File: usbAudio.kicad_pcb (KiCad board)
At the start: 2 copper layers, 34 parts, among them J2 USB_C_Receptacle_USB2.0_14P, J3 AudioJack3, SW1 PLAY/PAUSE, SW4 VOL+, SW5 VOL-, SW8 SW_SPDT, U1 PCM2706CPJTR, U4 MIC5504-3.3YM5-TR, Y2 Crystal_GND24

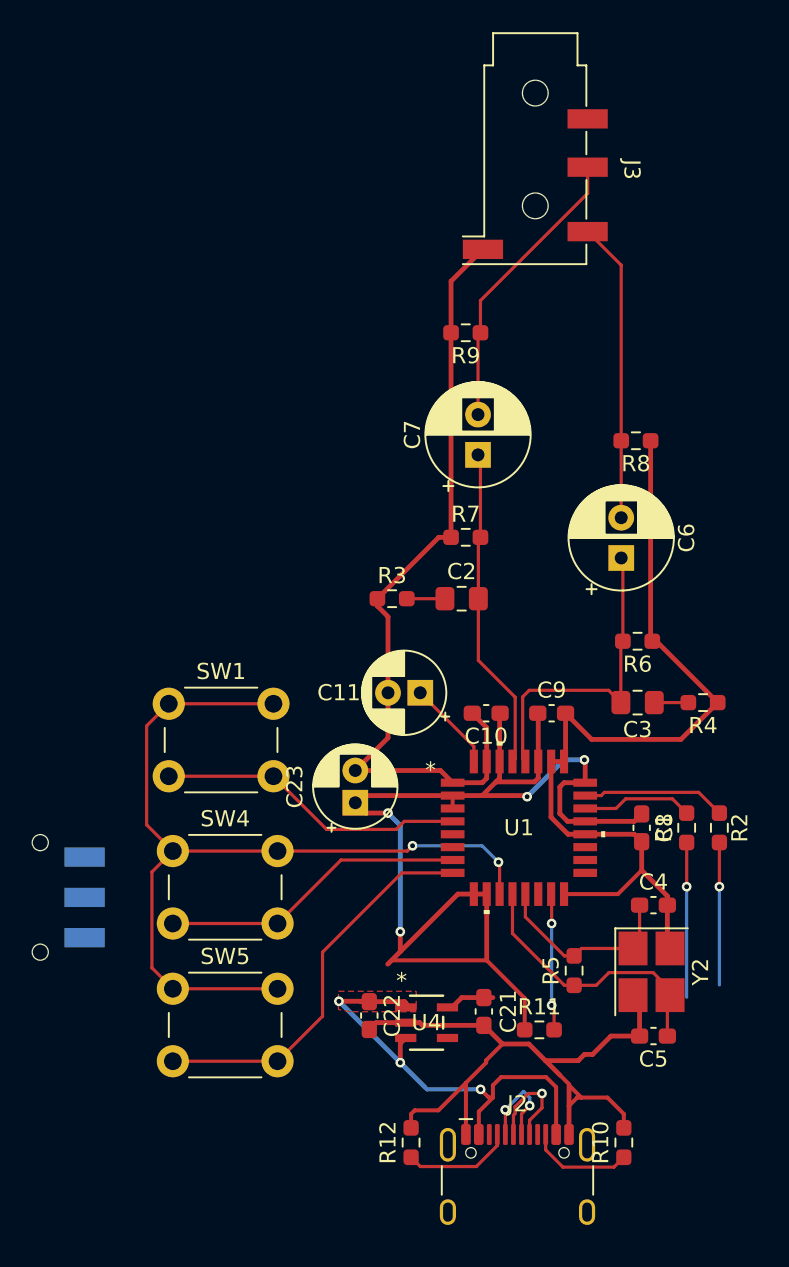
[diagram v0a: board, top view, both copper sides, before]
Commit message: Made ready for production!
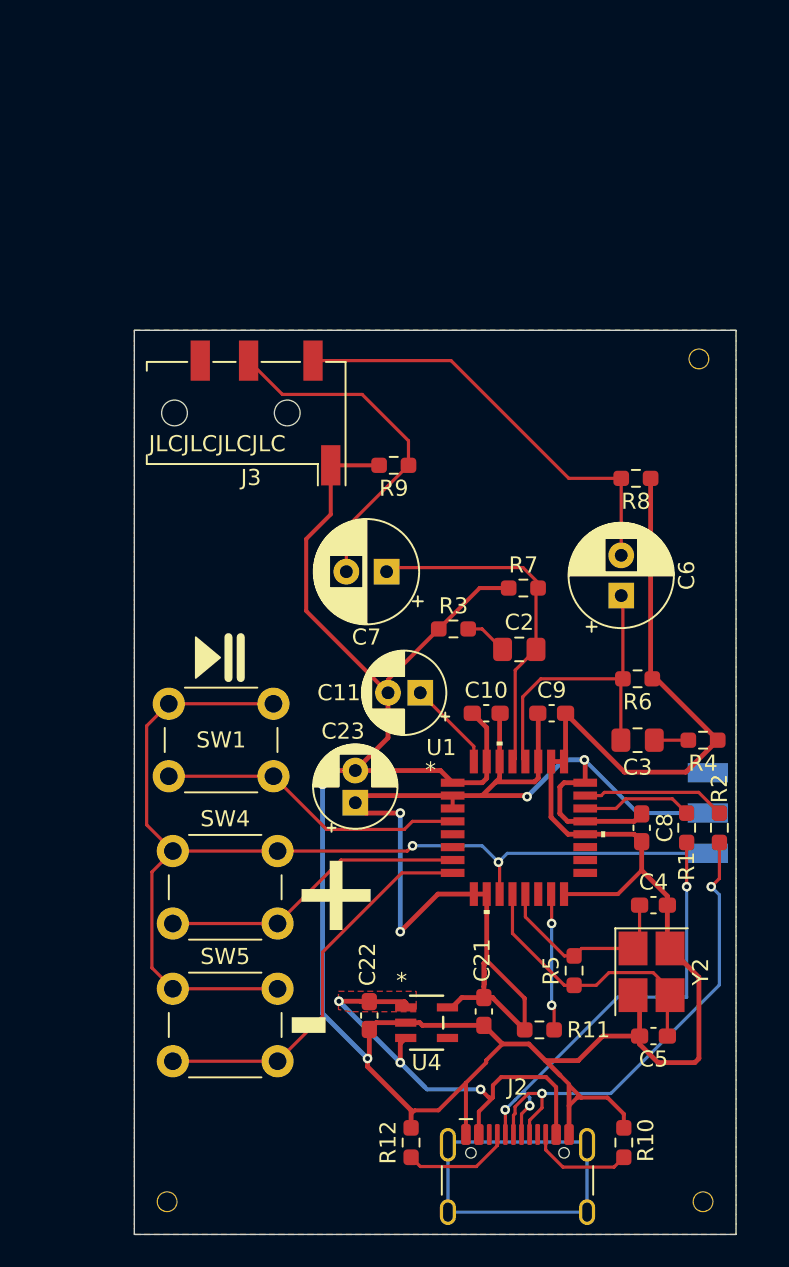
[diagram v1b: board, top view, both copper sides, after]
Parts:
- added G***: LOGO, LOGO, B.Cu at (141.4, 71.3)
- added G***: LOGO, LOGO, B.Cu at (126.0, 74.9)
- added G***: LOGO, LOGO, B.Cu at (141.0, 97.3)
- added REF**: PCBA tooling hole, JLCtooling:PCBA tooling hole, F.Cu at (119.4, 114.8)
- added REF**: PCBA tooling hole, JLCtooling:PCBA tooling hole, F.Cu at (152.4, 62.5)
- added REF**: PCBA tooling hole, JLCtooling:PCBA tooling hole, F.Cu at (152.7, 114.8)
- SW8: footprint JS102011SAQN:SW_JS102011SAQN -> JS102011SAQN:SW_JS102011SAQN_Xoverhang
- moved SW8 44.5 mm to (155.7, 90.7), turned to -90 degrees
- moved J3 23.2 mm to (124.6, 65.8), turned to 0 degrees
- moved R9 9.36 mm to (133.5, 69.1)
- moved C7 9.21 mm to (133.0, 75.7), turned to 180 degrees
- moved R7 4.77 mm to (141.5, 76.7)
- moved C2 4.77 mm to (141.2, 80.5)
- moved R3 4.25 mm to (137.2, 79.2)
- moved C3 2.33 mm to (148.6, 86.2)
- moved R4 2.33 mm to (152.7, 86.2)
- moved R8 2.33 mm to (148.5, 69.9)
- moved C6 2.33 mm to (147.6, 77.2)
- moved R6 2.33 mm to (148.6, 82.3)
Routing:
- net GND: track 149.2 -> 189.7 mm, vias 0 -> 2
- net unconnected-(J2-SHIELD-PadS1): track 0.00 -> 25.8 mm
- net Net-(J2-D+-PadA6): track 15.5 -> 29.7 mm
- net Suspend: track 55.8 -> 69.0 mm
- net Net-(J2-D--PadA7): track 15.8 -> 28.4 mm
- net /LeftOut: track 18.6 -> 26.9 mm
- net +3.3V: track 76.7 -> 82.3 mm
- net /RightOut: track 18.2 -> 21.7 mm
- net VoutR: track 20.2 -> 21.7 mm
- added copper zone on B.Cu, net +3.3V
- added copper zone on F.Cu, net +3.3V
- added copper zone on F.Cu, net GND
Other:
- board outline added: 37.4 x 56.1 mm
- board text added: "+"
- board text added: "-"
- board text added: "JLCJLCJLCJLC"
